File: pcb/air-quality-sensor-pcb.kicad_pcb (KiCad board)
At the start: 2 copper layers, 72.9 x 80.3 mm, 17 parts, among them J1 Conn_01x02, J2 Conn_02x04_Odd_Even, SW1 SW_Push_Dual, SW2 SW_DIP_x01, U1 XIAO-nRF52840-DIP, U2 Adafruit SGP40, U3 Adafruit SHT4X, U4 Adafruit BMP390, U5 Adafruit SCD4x

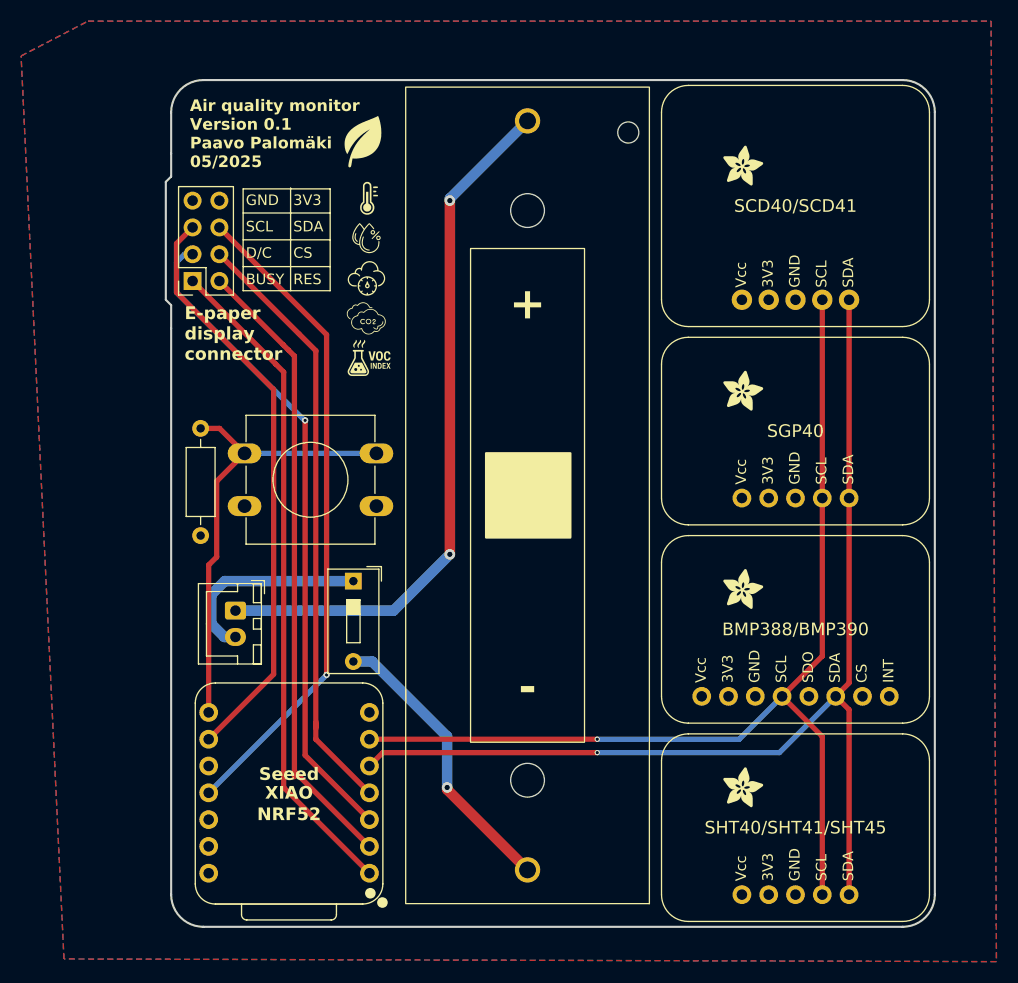
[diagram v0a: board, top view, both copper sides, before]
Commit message: New PCB design
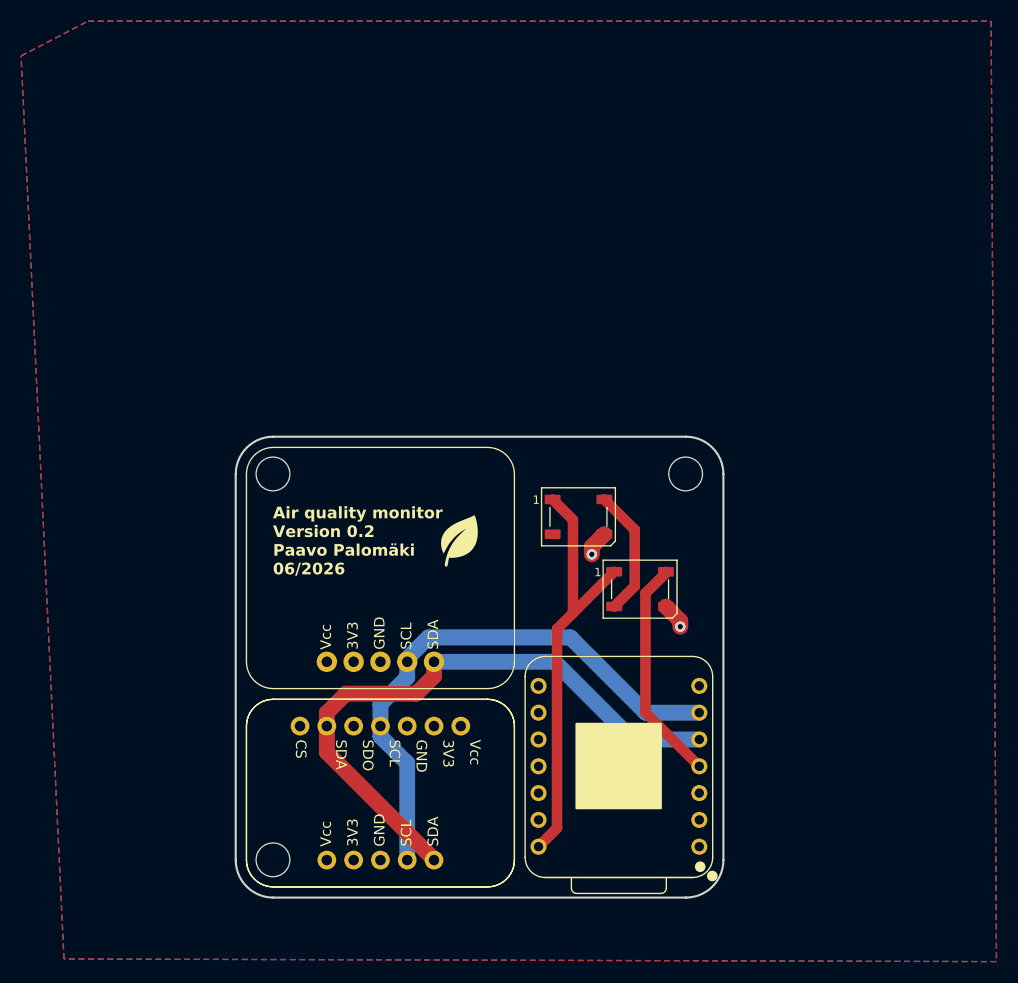
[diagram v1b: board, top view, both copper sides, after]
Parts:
- removed BT1: Battery_Cell, 18650_socket:18650_socket
- removed the G*** at (180.6, 68.6)
- removed the G*** at (180.8, 61.0)
- removed the G*** at (180.6, 72.4)
- removed the G*** at (180.6, 64.8)
- removed the G*** at (180.8, 76.2)
- removed J1: Conn_01x02, Connector_JST:JST_XH_B2B-XH-A_1x02_P2.50mm_Vertical
- removed J2: Conn_02x04_Odd_Even, Connector_PinSocket_2.54mm:PinSocket_2x04_P2.54mm_Vertical
- removed R1: R, Resistor_THT:R_Axial_DIN0207_L6.3mm_D2.5mm_P10.16mm_Horizontal
- removed SW1: SW_Push_Dual, Button_Switch_THT:SW_PUSH-12mm
- removed SW2: SW_DIP_x01, Button_Switch_THT:SW_DIP_SPSTx01_Slide_9.78x4.72mm_W7.62mm_P2.54mm
- removed U4: Adafruit BMP390, adafruit_bmp390:adafruit_bmp390
- added D1: WS2812B, LED_SMD:LED_WS2812B_PLCC4_5.0x5.0mm_P3.2mm, F.Cu at (206.5, 98.0)
- added D2: WS2812B, LED_SMD:LED_WS2812B_PLCC4_5.0x5.0mm_P3.2mm, F.Cu at (200.7, 91.2)
- added H1: MountingHole, MountingHole:MountingHole_3.2mm_M3, F.Cu at (210.8, 87.1)
- added H2: MountingHole, MountingHole:MountingHole_3.2mm_M3, F.Cu at (171.7, 123.7)
- added H3: MountingHole, MountingHole:MountingHole_3.2mm_M3, F.Cu at (171.7, 87.1)
- U1: footprint seeed_xiao_nrf52:XIAO-nRF52840-DIP2 -> Seeed_XIAO_nRF52840:XIAO-nRF52840-DIP
- U2: value Adafruit SGP40 -> Adafruit BME680; footprint adafruit_sgp40:adafruit_sgp40 -> adafruit_bme680:adafruit_bme680
- moved U2 52.2 mm to (181.9, 117.4), turned to 180 degrees
- moved U5 52.2 mm to (181.9, 96.0)
- moved U3 39.5 mm to (181.9, 117.4)
- moved G*** 38.9 mm to (189.2, 93.5)
- moved U1 31.4 mm to (204.5, 114.8)
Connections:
- U1 pad 1: EPD_BUSY -> unconnected-(U1-P0.02_AIN0_LOW_A0_D0-Pad1)
- U1 pad 14: unconnected-(U1-VBUS-Pad14) -> VBUS
- U1 pad 2: EPD_RES -> unconnected-(U1-P0.03_AIN1_LOW_A1_D1-Pad2)_1
- U1 pad 3: EPD D/C -> unconnected-(U1-P0.28_AIN4_LOW_A2_D2-Pad3)
- U1 pad 4: EPD CS -> LED_DI
- U2 pad 5: I2C_SDA -> unconnected-(U2-SDO-Pad5)
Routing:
- net Net-(BT1--): track 66.7 -> 0.00 mm, vias 2 -> 0
- net EPD_BUSY: track 63.1 -> 0.00 mm
- net SPI_SDA: track 62.4 -> 0.00 mm, vias 1 -> 0
- net EPD D/C: track 62.3 -> 0.00 mm, vias 1 -> 0
- net EPD_RES: track 60.0 -> 0.00 mm
- net EPD CS: track 57.5 -> 0.00 mm
- net SPI_SCL: track 55.5 -> 0.00 mm
- net I2C_SCL: track 100.3 -> 52.7 mm, vias 1 -> 0
- net I2C_SDA: track 104.4 -> 59.3 mm, vias 1 -> 0
- net Button: track 43.6 -> 0.00 mm
- net VBUS: track 0.00 -> 40.6 mm
- net Net-(BT1-+): track 27.8 -> 0.00 mm, vias 1 -> 0
- net LED_DI: track 0.00 -> 21.4 mm
- net Net-(J1-Pin_2): track 19.6 -> 0.00 mm
- net Net-(D1-DOUT): track 0.00 -> 12.2 mm
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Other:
- board size 72.9 x 80.3 mm -> 46.2 x 43.7 mm
- board text added: "Air quality monitor Version 0.2 Paavo Palomäki 06/2026"
- board text removed: "3V3"
- board text removed: "Air quality monitor Version 0.1 Paavo Palomäki 05/2025"
- board text removed: "BUSY"
- board text removed: "CS"
- board text removed: "D/C"
- board text removed: "E-paper display connector"
- board text removed: "GND"
- board text removed: "RES"
- board text removed: "SCL"
- board text removed: "SDA"
